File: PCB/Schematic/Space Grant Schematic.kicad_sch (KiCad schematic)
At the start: 4 parts, among them J1 Raspberry_Pi_4, U1 L298N, U2 L298N

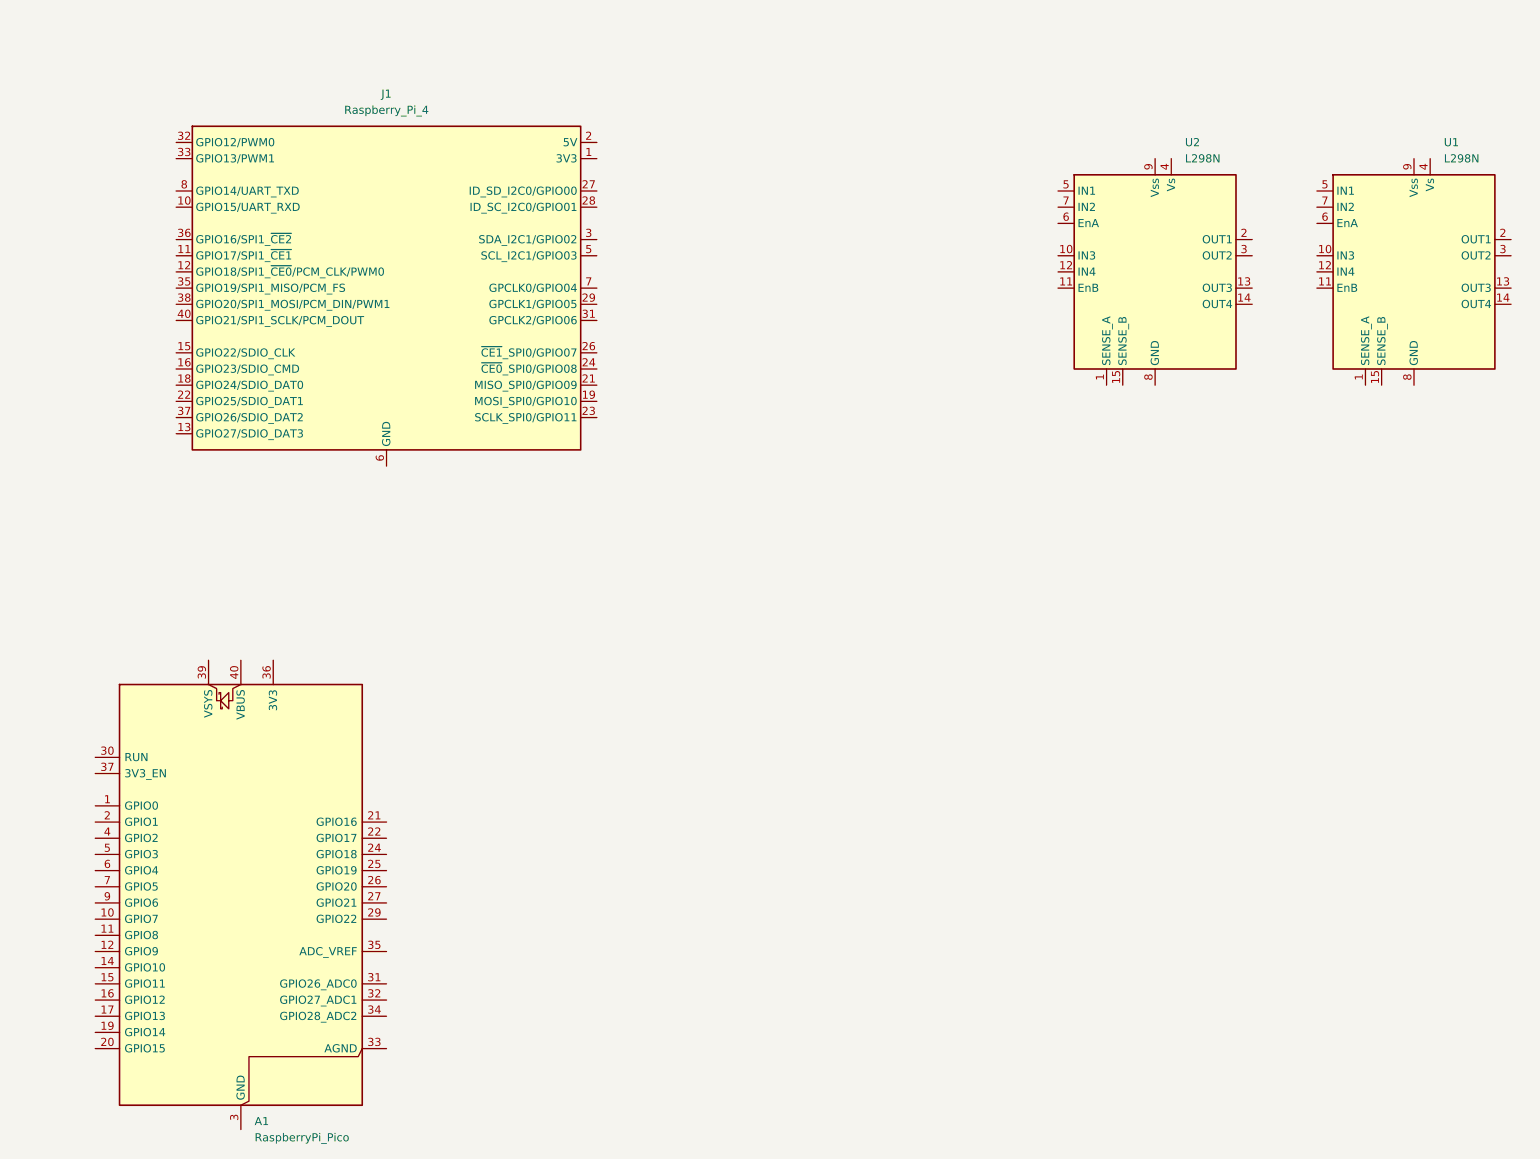
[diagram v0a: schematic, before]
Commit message: Some of my stuff
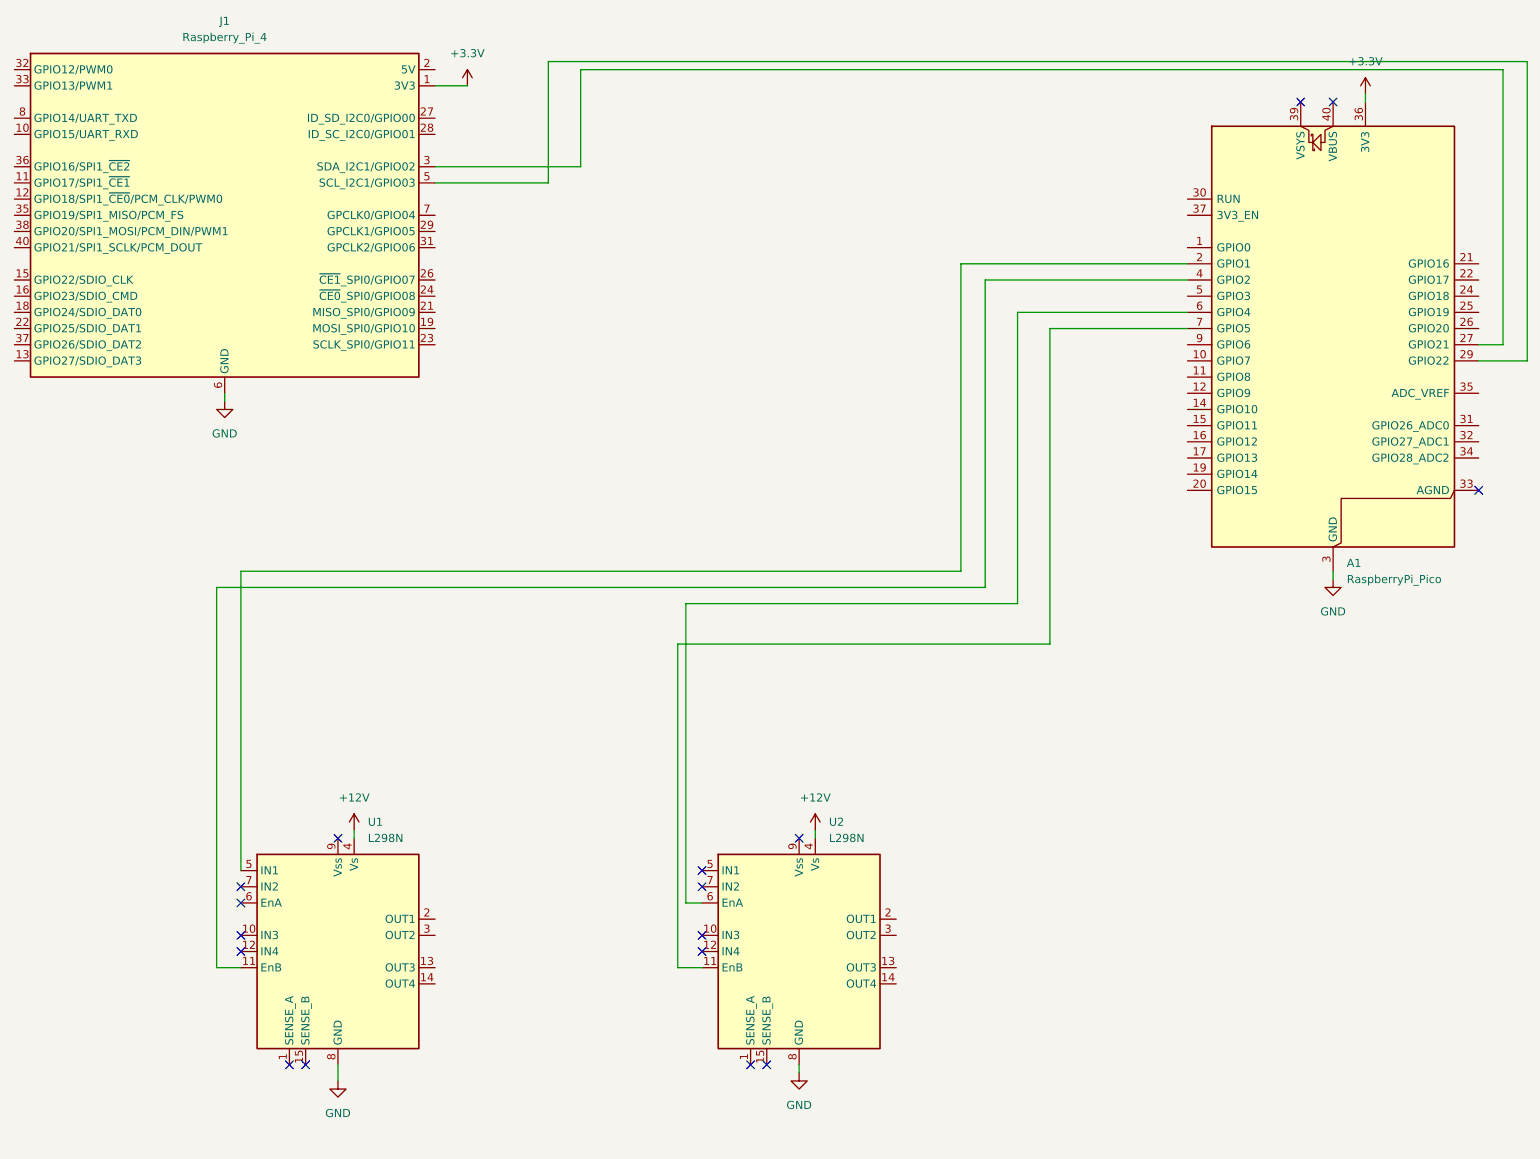
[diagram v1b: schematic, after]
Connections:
- net GND: now reaches A1.13 (GND), A1.18 (GND), A1.23 (GND), A1.28 (GND), A1.3 (GND), A1.38 (GND), A1.8 (GND)
- net GND: now also J1.14 (GND), J1.20 (GND), J1.25 (GND), J1.30 (GND), J1.34 (GND), J1.39 (GND), J1.6 (GND), J1.9 (GND), U1.8 (GND), U2.8 (GND)
- net at A1.2 (GPIO1): now also U1.5 (IN1)
- net at A1.27 (GPIO21): now also J1.3 (SDA_I2C1/GPIO02)
- net at A1.29 (GPIO22): now also J1.5 (SCL_I2C1/GPIO03)
- net +3.3V: now reaches A1.36 (3V3)
- net +3.3V: now also J1.1 (3V3), J1.17 (3V3)
- net at A1.4 (GPIO2): now also U1.11 (EnB)
- net at A1.6 (GPIO4): now also U2.6 (EnA)
- net at A1.7 (GPIO5): now also U2.11 (EnB)
- net +12V: now reaches U2.4 (Vs)
- net +12V: now also U1.4 (Vs)
- no-connect marks 0 -> 17
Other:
- moved on the sheet: A1, J1, U1, U2
